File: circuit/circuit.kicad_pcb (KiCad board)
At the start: 2 copper layers, 33 x 33 mm, 3 parts

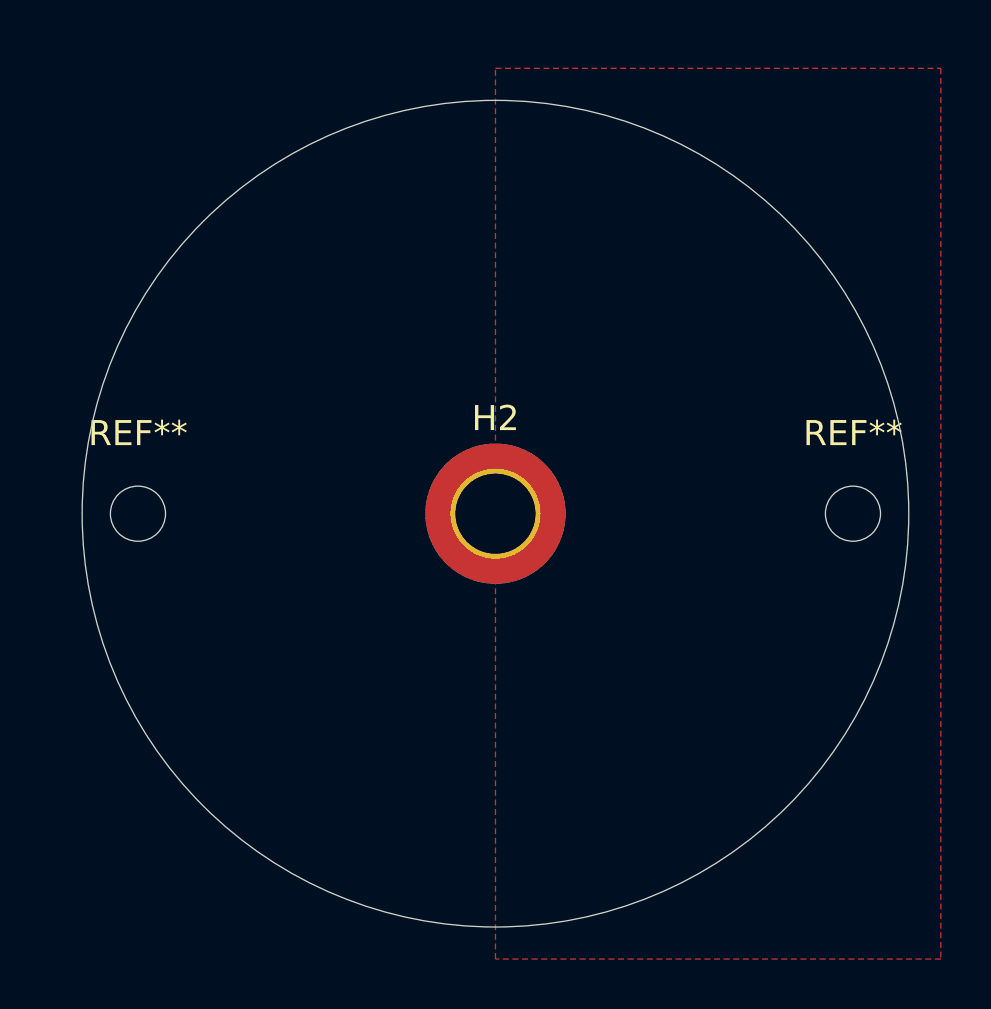
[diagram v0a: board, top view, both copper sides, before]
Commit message: making some improvements to the end circuit
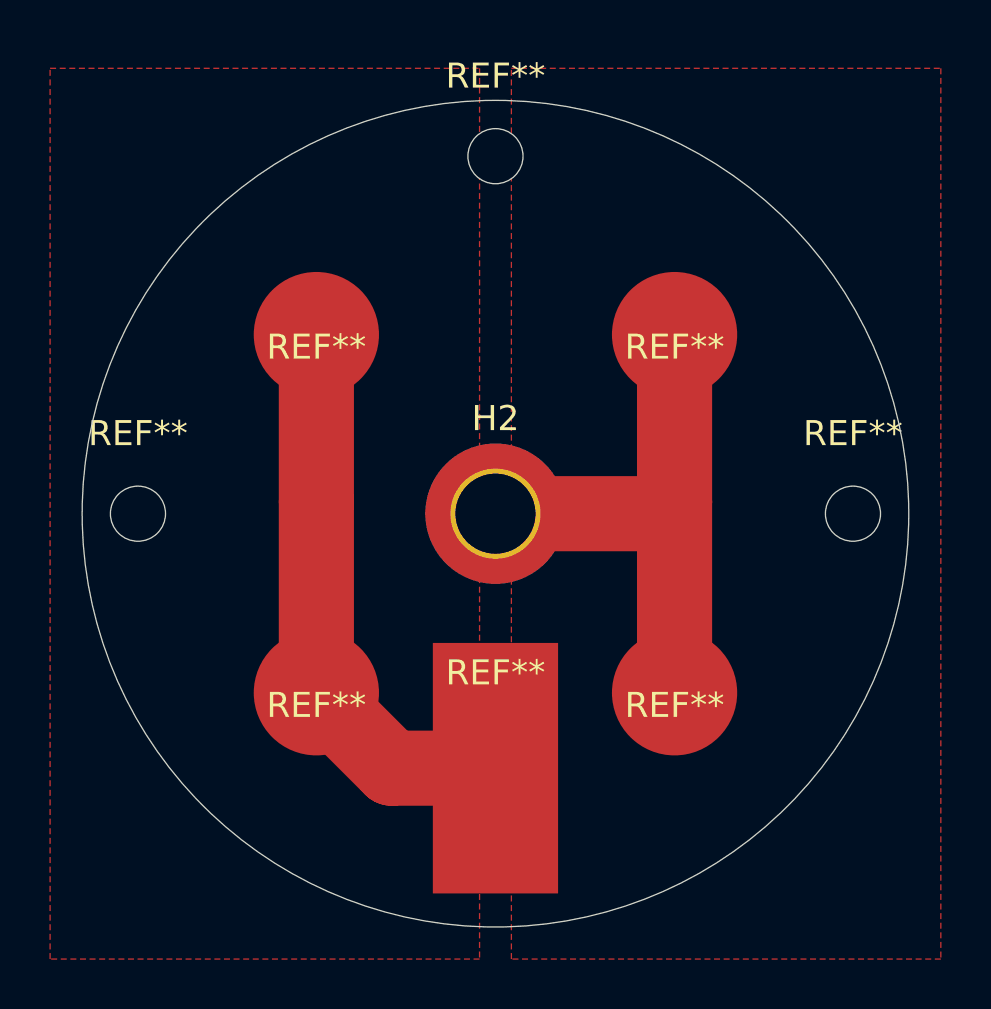
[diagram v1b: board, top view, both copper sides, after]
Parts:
- added REF**: Pad_5mm, Pad_5mm, F.Cu at (184.9, 96.0)
- added REF**: Pad_5mm, Pad_5mm, F.Cu at (184.9, 81.8)
- added REF**: Pad_5mm, Pad_5mm, F.Cu at (170.7, 96.0)
- added REF**: Pad_5mm, Pad_5mm, F.Cu at (170.7, 81.8)
- added REF**: MountingHole_2.2mm_M2, MountingHole:MountingHole_2.2mm_M2, F.Cu at (177.8, 74.6)
- added REF**: SolderWirePad_1x01_SMD_5x10mm, Connector_Wire:SolderWirePad_1x01_SMD_5x10mm, F.Cu at (177.8, 99.1)
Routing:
- net VSS: track 0.00 -> 22.7 mm
- net GND: track 0.00 -> 21.6 mm
- added copper zone on F.Cu, net VSS
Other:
- net class power added: clearance 0.2, trace_width 3, via_dia 0.8, via_drill 0.4
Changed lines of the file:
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@@
   (general
     (thickness 1.6)
-    (drawings 1)
-    (tracks 0)
+    (drawings 5)
+    (tracks 8)
     (zones 0)
-    (modules 3)
-    (nets 2)
+    (modules 9)
+    (nets 3)
   )
   (page A4)
@@
     (last_trace_width 0.25)
     (trace_clearance 0.2)
-    (zone_clearance 0.508)
+    (zone_clearance 1)
     (zone_45_only no)
     (trace_min 0.2)
@@
     (mod_text_size 1 1)
     (mod_text_width 0.15)
-    (pad_size 1.524 1.524)
-    (pad_drill 0.762)
+    (pad_size 5 5)
+    (pad_drill 0)
     (pad_to_mask_clearance 0)
     (aux_axis_origin 0 0)
     (visible_elements FFFFFF7F)
     (pcbplotparams
-      (layerselection 0x010fc_ffffffff)
+      (layerselection 0x01000_ffffffff)
       (usegerberextensions false)
       (usegerberattributes true)
@@
       (outputformat 1)
       (mirror false)
-      (drillshape 1)
+      (drillshape 0)
       (scaleselection 1)
-      (outputdirectory ""))
+      (outputdirectory "output_files/"))
   )
   (net 0 "")
   (net 1 GND)
+  (net 2 VSS)
   (net_class Default "This is the default net class."
     (clearance 0.2)
@@
     (uvia_dia 0.3)
     (uvia_drill 0.1)
+  )
+  (net_class power ""
+    (clearance 0.2)
+    (trace_width 3)
+    (via_dia 0.8)
+    (via_drill 0.4)
+    (uvia_dia 0.3)
+    (uvia_drill 0.1)
     (add_net GND)
+    (add_net VSS)
+  )
+  (module Pad_5mm (layer F.Cu)
+    (at 184.95 96.05)
+    (fp_text reference REF** (at 0 0.5) (layer F.SilkS)
+      (effects (font (size 1 1) (thickness 0.15)))
+    )
+    (fp_text value Pad_5mm (at 0 -0.5) (layer F.Fab)
+      (effects (font (size 1 1) (thickness 0.15)))
+    )
+    (pad 1 smd circle (at 0 0) (size 5 5) (layers F.Cu F.Paste F.Mask)
+      (net 1 GND))
+  )
+  (module Pad_5mm (layer F.Cu)
+    (at 184.95 81.75)
+    (fp_text reference REF** (at 0 0.5) (layer F.SilkS)
+      (effects (font (size 1 1) (thickness 0.15)))
+    )
+    (fp_text value Pad_5mm (at 0 -0.5) (layer F.Fab)
+      (effects (font (size 1 1) (thickness 0.15)))
+    )
+    (pad 1 smd circle (at 0 0) (size 5 5) (layers F.Cu F.Paste F.Mask)
+      (net 1 GND))
+  )
+  (module Pad_5mm (layer F.Cu)
+    (at 170.65 96.05)
+    (fp_text reference REF** (at 0 0.5) (layer F.SilkS)
+      (effects (font (size 1 1) (thickness 0.15)))
+    )
+    (fp_text value Pad_5mm (at 0 -0.5) (layer F.Fab)
+      (effects (font (size 1 1) (thickness 0.15)))
+    )
+    (pad 1 smd circle (at 0 0) (size 5 5) (layers F.Cu F.Paste F.Mask)
+      (net 2 VSS))
+  )
+  (module Pad_5mm (layer F.Cu)
+    (at 170.65 81.75)
+    (fp_text reference REF** (at 0 0.5) (layer F.SilkS)
+      (effects (font (size 1 1) (thickness 0.15)))
+    )
+    (fp_text value Pad_5mm (at 0 -0.5) (layer F.Fab)
+      (effects (font (size 1 1) (thickness 0.15)))
+    )
+    (pad 1 smd circle (at 0 0) (size 5 5) (layers F.Cu F.Paste F.Mask)
+      (net 2 VSS))
+  )
+  (module MountingHole:MountingHole_2.2mm_M2 (layer F.Cu)
+    (at 177.8 74.6276)
+    (descr "Mounting Hole 2.2mm, no annular, M2")
+    (tags "mounting hole 2.2mm no annular m2")
+    (attr virtual)
+    (fp_text reference REF** (at 0 -3.2) (layer F.SilkS)
+      (effects (font (size 1 1) (thickness 0.15)))
+    )
+    (fp_text value MountingHole_2.2mm_M2 (at 0 3.2) (layer F.Fab)
+      (effects (font (size 1 1) (thickness 0.15)))
+    )
+    (fp_text user %R (at 0.3 0) (layer F.Fab)
+      (effects (font (size 1 1) (thickness 0.15)))
+    )
+    (fp_circle (center 0 0) (end 2.2 0) (layer Cmts.User) (width 0.15))
+    (fp_circle (center 0 0) (end 2.45 0) (layer F.CrtYd) (width 0.05))
+    (pad 1 np_thru_hole circle (at 0 0) (size 2.2 2.2) (drill 2.2) (layers *.Cu *.Mask))
+  )
+  (module Connector_Wire:SolderWirePad_1x01_SMD_5x10mm (layer F.Cu)
+    (at 177.8 99.06)
+    (descr "Wire Pad, Square, SMD Pad,  5mm x 10mm,")
+    (tags "MesurementPoint Square SMDPad 5mmx10mm ")
+    (attr smd virtual)
+    (fp_text reference REF** (at 0 -3.81) (layer F.SilkS)
+      (effects (font (size 1 1) (thickness 0.15)))
+    )
+    (fp_text value SolderWirePad_1x01_SMD_5x10mm (at 0 6.35) (layer F.Fab)
+      (effects (font (size 1 1) (thickness 0.15)))
+    )
+    (fp_text user %R (at 0 0) (layer F.Fab)
+      (effects (font (size 1 1) (thickness 0.15)))
+    )
+    (fp_line (start 2.75 -5.25) (end -2.75 -5.25) (layer F.CrtYd) (width 0.05))
+    (fp_line (start 2.75 5.25) (end 2.75 -5.25) (layer F.CrtYd) (width 0.05))
+    (fp_line (start -2.75 5.25) (end 2.75 5.25) (layer F.CrtYd) (width 0.05))
+    (fp_line (start -2.75 -5.25) (end -2.75 5.25) (layer F.CrtYd) (width 0.05))
+    (pad 1 smd rect (at 0 0) (size 5 10) (layers F.Cu F.Paste F.Mask)
+      (net 2 VSS))
   )
   (module MountingHole:MountingHole_2.2mm_M2 (layer F.Cu)
@@
       (effects (font (size 1 1) (thickness 0.15)))
     )
+    (fp_circle (center 0 0) (end 2.45 0) (layer F.CrtYd) (width 0.05))
+    (fp_circle (center 0 0) (end 2.2 0) (layer Cmts.User) (width 0.15))
     (fp_text user %R (at 2.8424 0) (layer F.Fab)
       (effects (font (size 1 1) (thickness 0.15)))
     )
-    (fp_circle (center 0 0) (end 2.2 0) (layer Cmts.User) (width 0.15))
-    (fp_circle (center 0 0) (end 2.45 0) (layer F.CrtYd) (width 0.05))
     (pad 1 np_thru_hole circle (at 0 0) (size 2.2 2.2) (drill 2.2) (layers *.Cu *.Mask))
   )
@@
       (effects (font (size 1 1) (thickness 0.15)))
     )
+    (fp_circle (center 0 0) (end 2.45 0) (layer F.CrtYd) (width 0.05))
+    (fp_circle (center 0 0) (end 2.2 0) (layer Cmts.User) (width 0.15))
     (fp_text user %R (at 0.3 0) (layer F.Fab)
       (effects (font (size 1 1) (thickness 0.15)))
     )
-    (fp_circle (center 0 0) (end 2.2 0) (layer Cmts.User) (width 0.15))
-    (fp_circle (center 0 0) (end 2.45 0) (layer F.CrtYd) (width 0.05))
     (pad 1 np_thru_hole circle (at 0 0) (size 2.2 2.2) (drill 2.2) (layers *.Cu *.Mask))
   )
@@
       (effects (font (size 1 1) (thickness 0.15)))
     )
+    (fp_circle (center 0 0) (end 3.05 0) (layer F.CrtYd) (width 0.05))
+    (fp_circle (center 0 0) (end 2.8 0) (layer Cmts.User) (width 0.15))
     (fp_text user %R (at 0.3 0) (layer F.Fab)
       (effects (font (size 1 1) (thickness 0.15)))
     )
-    (fp_circle (center 0 0) (end 2.8 0) (layer Cmts.User) (width 0.15))
-    (fp_circle (center 0 0) (end 3.05 0) (layer F.CrtYd) (width 0.05))
     (pad 1 connect circle (at 0 0) (size 5.6 5.6) (layers B.Cu B.Mask)
       (net 1 GND))
@@
       (net 1 GND))
   )
+  (gr_circle (center 170.65 96.05) (end 175.65 96.05) (layer Dwgs.User) (width 0.15))
+  (gr_circle (center 170.65 81.75) (end 175.65 81.75) (layer Dwgs.User) (width 0.15))
+  (gr_circle (center 184.95 81.75) (end 189.95 81.75) (layer Dwgs.User) (width 0.15))
+  (gr_circle (center 184.95 96.05) (end 189.95 96.05) (layer Dwgs.User) (width 0.15))
   (gr_circle (center 177.8 88.9) (end 194.3 88.9) (layer Edge.Cuts) (width 0.05))
+  (segment (start 184.48 88.9) (end 184.95 88.43) (width 3) (layer F.Cu) (net 1))
+  (segment (start 177.8 88.9) (end 184.48 88.9) (width 3) (layer F.Cu) (net 1))
+  (segment (start 184.95 88.43) (end 184.95 96.05) (width 3) (layer F.Cu) (net 1))
+  (segment (start 184.95 81.75) (end 184.95 88.43) (width 3) (layer F.Cu) (net 1))
+  (segment (start 170.65 81.75) (end 170.65 88.43) (width 3) (layer F.Cu) (net 2))
+  (segment (start 170.65 88.43) (end 170.65 96.05) (width 3) (layer F.Cu) (net 2))
+  (segment (start 173.66 99.06) (end 170.65 96.05) (width 3) (layer F.Cu) (net 2))
+  (segment (start 177.8 99.06) (end 173.66 99.06) (width 3) (layer F.Cu) (net 2))
   (zone (net 1) (net_name GND) (layer F.Cu) (hatch edge 0.508)
-    (connect_pads yes (clearance 0.508))
+    (priority 1)
+    (connect_pads no (clearance 1))
     (min_thickness 1)
-    (fill yes (arc_segments 32) (thermal_gap 0.508) (thermal_bridge_width 2))
+    (fill yes (arc_segments 32) (thermal_gap 1) (thermal_bridge_width 3))
     (polygon
       (pts
-        (xy 195.58 106.68) (xy 177.8 106.68) (xy 177.8 71.12) (xy 195.58 71.12)
+        (xy 195.58 106.68) (xy 178.435 106.68) (xy 178.435 71.12) (xy 195.58 71.12)
       )
     )
+  )
+  (zone (net 2) (net_name VSS) (layer F.Cu) (hatch edge 0.508)
+    (priority 1)
+    (connect_pads no (clearance 1))
+    (min_thickness 1)
+    (fill yes (arc_segments 32) (thermal_gap 1) (thermal_bridge_width 3))
+    (polygon
+      (pts
+        (xy 177.165 106.68) (xy 160.02 106.68) (xy 160.02 71.12) (xy 177.165 71.12)
+      )
+    )
